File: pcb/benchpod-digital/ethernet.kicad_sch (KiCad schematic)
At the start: 42 parts, among them J7 HR911105A_C12074, U6 LAN8742AI-CZ-TR, Y1 6pF ±10ppm SMD2016-4P Crystal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

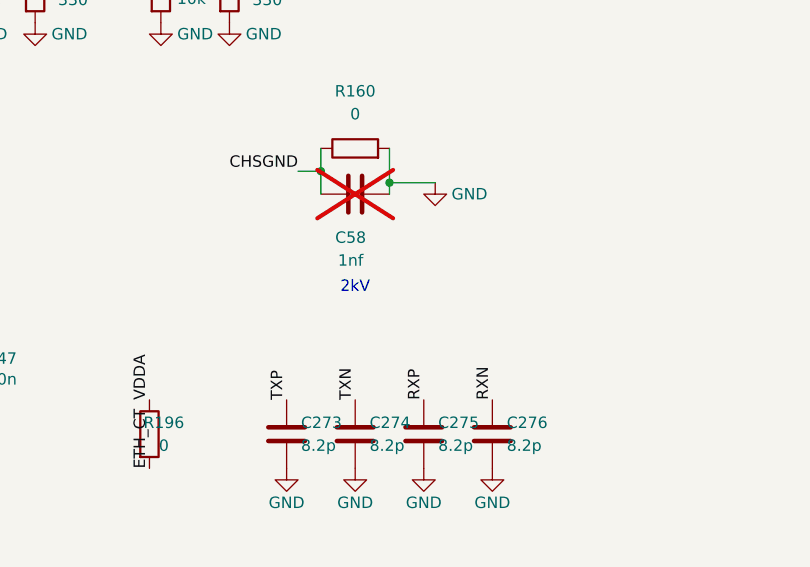
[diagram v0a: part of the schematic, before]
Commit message: signal filtering / improvement
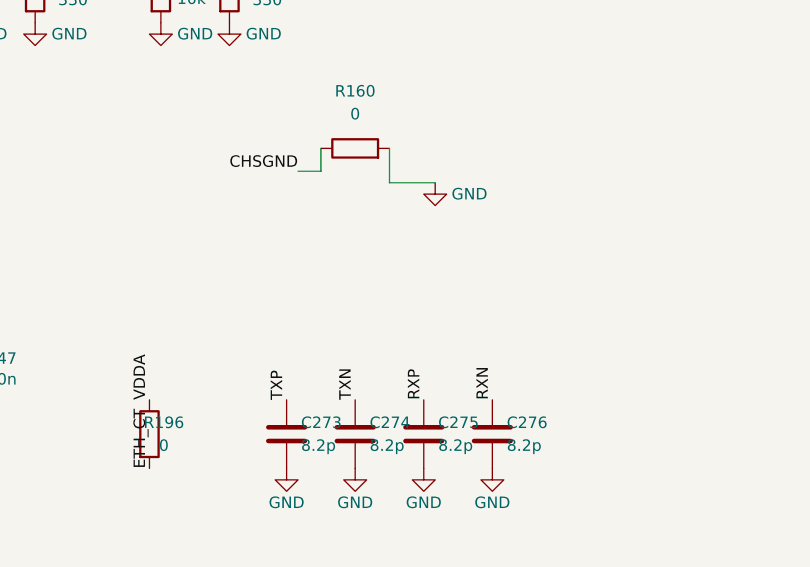
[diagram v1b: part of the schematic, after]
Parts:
- removed C58: 1nf, Capacitor_SMD:C_1206_3216Metric, symbol Device:C
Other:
- note removed: "2kV"
